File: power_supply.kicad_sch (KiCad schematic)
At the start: 8 parts

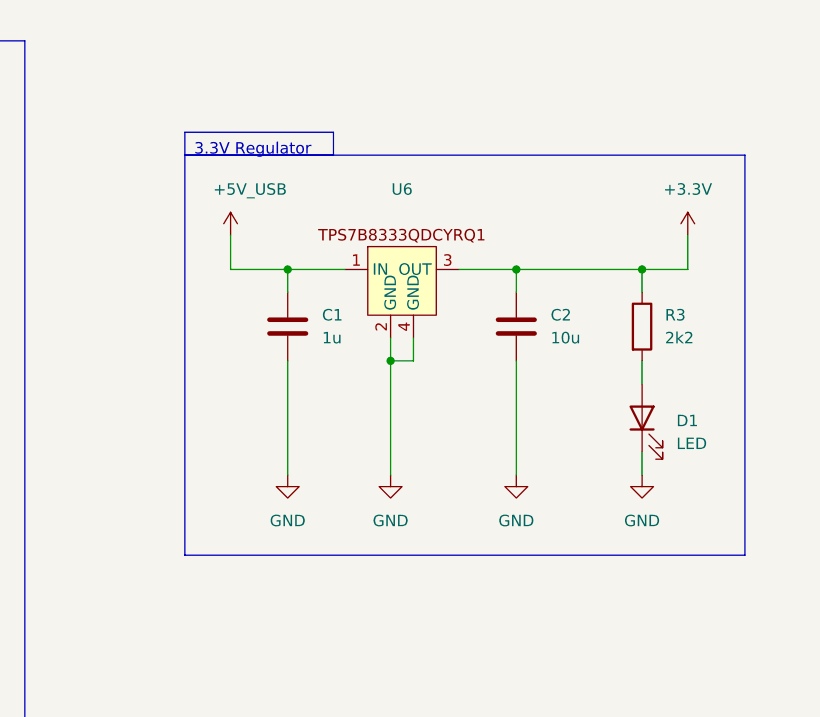
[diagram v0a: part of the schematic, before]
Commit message: dasda
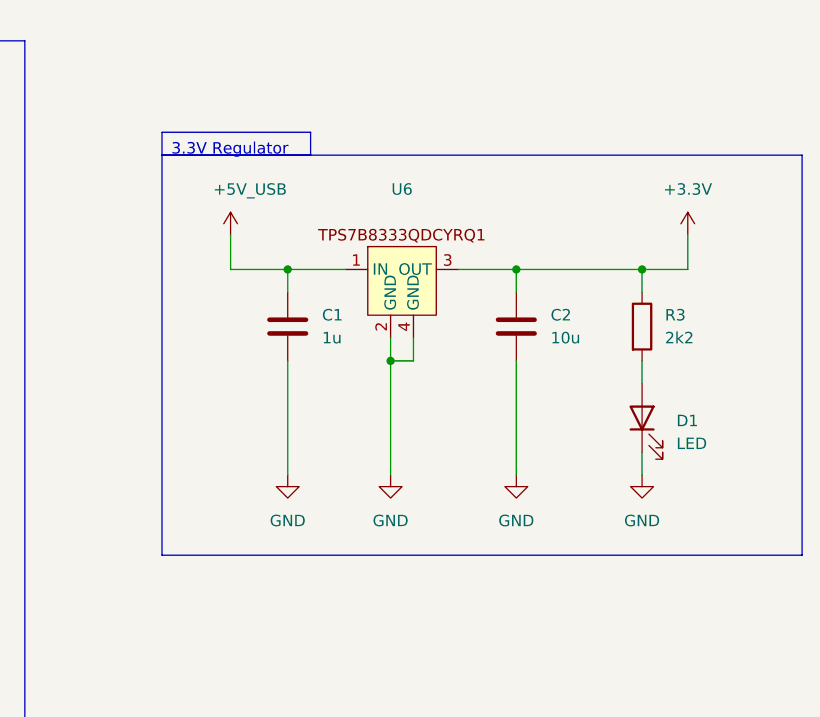
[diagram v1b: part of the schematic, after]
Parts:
- C1, C2: footprint (none) -> Capacitor_SMD:C_0201_0603Metric
- D1: footprint (none) -> LED_THT:LED_D3.0mm
- R1, R2, R3: footprint (none) -> Resistor_SMD:R_0201_0603Metric
- U4: footprint (none) -> custom:UJ20-C-H-C-MSMT-TR
- U6: footprint (none) -> custom:TPS7B8333QDCYRQ1
